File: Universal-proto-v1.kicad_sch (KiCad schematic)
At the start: 44 parts, among them J1 Bus_ISA_8bit, J2 ISA Breakout, J3 Pico GPIO Breakout

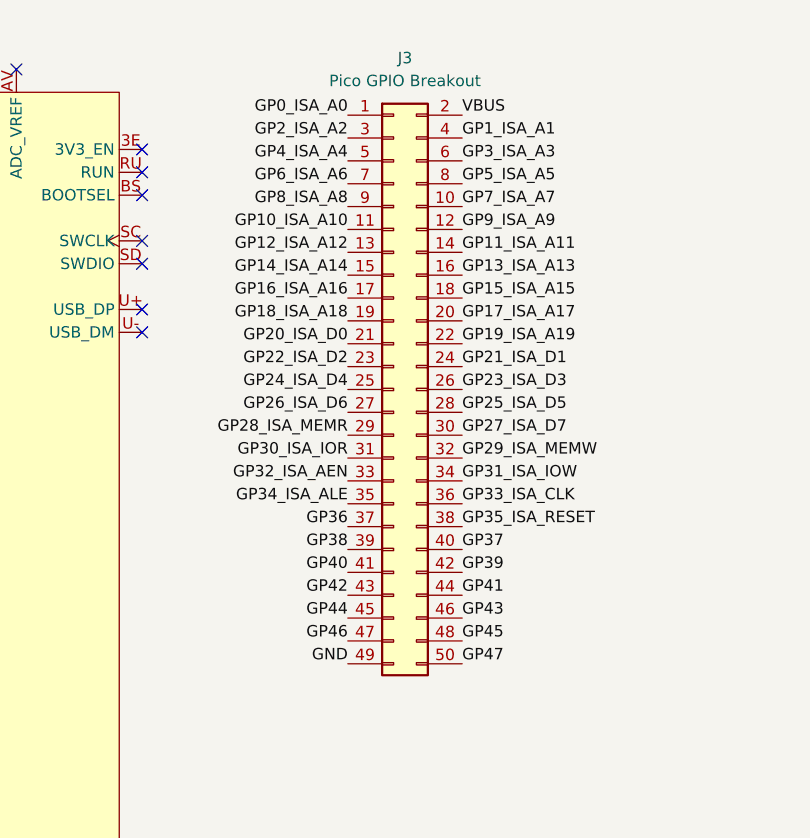
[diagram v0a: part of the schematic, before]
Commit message: Pre-split of GPIO breakout
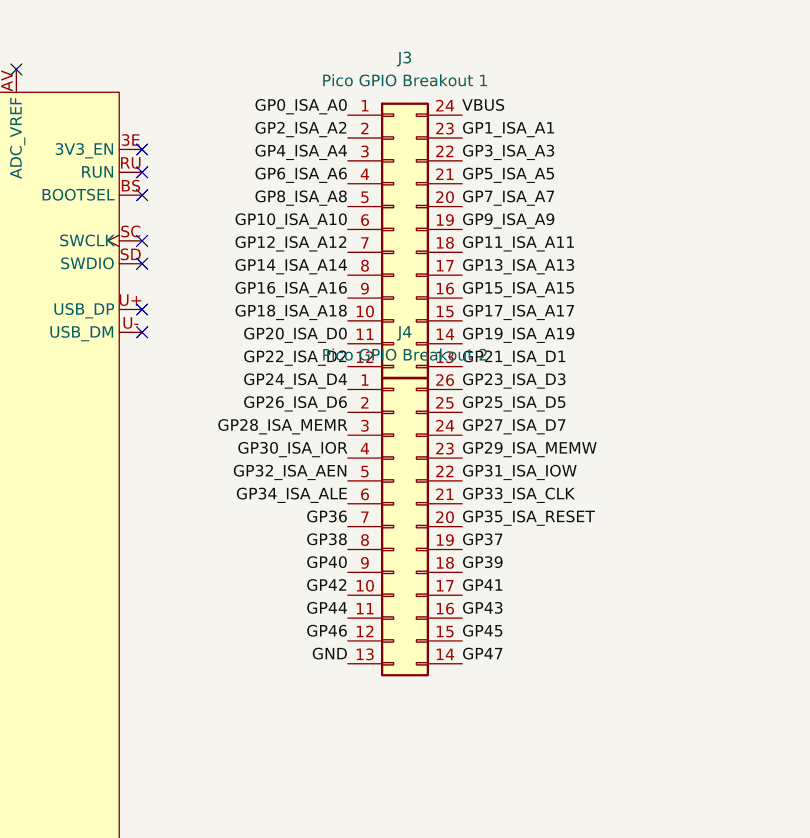
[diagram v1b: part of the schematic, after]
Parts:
- removed J3: Pico GPIO Breakout, Connector_PinHeader_2.54mm:PinHeader_2x25_P2.54mm_Vertical, symbol Connector_Generic:Conn_02x25_Odd_Even
- added J3: Pico GPIO Breakout 1, symbol Connector_Generic:Conn_02x12_Counter_Clockwise
- added J4: Pico GPIO Breakout 2, symbol Connector_Generic:Conn_02x13_Counter_Clockwise
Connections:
- net GND: now also J4.13 (Pin_13)
- net GP0_ISA_A0: now also J3.1 (Pin_1)
- net GP10_ISA_A10: now also J3.6 (Pin_6)
- net GP11_ISA_A11: now also J3.18 (Pin_18)
- net GP12_ISA_A12: now also J3.7 (Pin_7)
- net GP13_ISA_A13: now also J3.17 (Pin_17)
- net GP14_ISA_A14: now also J3.8 (Pin_8)
- net GP15_ISA_A15: now also J3.16 (Pin_16)
- net GP16_ISA_A16: now also J3.9 (Pin_9)
- net GP17_ISA_A17: now also J3.15 (Pin_15)
- net GP18_ISA_A18: now also J3.10 (Pin_10)
- net GP19_ISA_A19: now also J3.14 (Pin_14)
- net GP1_ISA_A1: now also J3.23 (Pin_23)
- net GP20_ISA_D0: now also J3.11 (Pin_11)
- net GP21_ISA_D1: now also J3.13 (Pin_13)
- net GP22_ISA_D2: now also J3.12 (Pin_12)
- net GP23_ISA_D3: now also J4.26 (Pin_26)
- net GP24_ISA_D4: now also J4.1 (Pin_1)
- net GP25_ISA_D5: now also J4.25 (Pin_25)
- net GP26_ISA_D6: now also J4.2 (Pin_2)
- net GP27_ISA_D7: now also J4.24 (Pin_24)
- net GP28_ISA_MEMR: now also J4.3 (Pin_3)
- net GP29_ISA_MEMW: now also J4.23 (Pin_23)
- net GP2_ISA_A2: now also J3.2 (Pin_2)
- net GP30_ISA_IOR: now also J4.4 (Pin_4)
- net GP31_ISA_IOW: now also J4.22 (Pin_22)
- net GP32_ISA_AEN: now also J4.5 (Pin_5)
- net GP33_ISA_CLK: now also J4.21 (Pin_21)
- net GP34_ISA_ALE: now also J4.6 (Pin_6)
- net GP35_ISA_RESET: now also J4.20 (Pin_20)
- net GP36: now also J4.7 (Pin_7)
- net GP37: now also J4.19 (Pin_19)
- net GP38: now also J4.8 (Pin_8)
- net GP39: now also J4.18 (Pin_18)
- net GP3_ISA_A3: now also J3.22 (Pin_22)
- net GP40: now also J4.9 (Pin_9)
- net GP41: now also J4.17 (Pin_17)
- net GP42: now also J4.10 (Pin_10)
- net GP43: now also J4.16 (Pin_16)
- net GP44: now also J4.11 (Pin_11)
- net GP45: now also J4.15 (Pin_15)
- net GP46: now also J4.12 (Pin_12)
- net GP47: now also J4.14 (Pin_14)
- net GP4_ISA_A4: now also J3.3 (Pin_3)
- net GP5_ISA_A5: now also J3.21 (Pin_21)
- net GP6_ISA_A6: now also J3.4 (Pin_4)
- net GP7_ISA_A7: now also J3.20 (Pin_20)
- net GP8_ISA_A8: now also J3.5 (Pin_5)
- net GP9_ISA_A9: now also J3.19 (Pin_19)
- net VBUS: now also J3.24 (Pin_24)
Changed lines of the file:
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@@
 	)
 	(symbol
+		(lib_id "Connector_Generic:Conn_02x13_Counter_Clockwise")
+		(at 229.87 71.12 0)
+		(unit 1)
+		(exclude_from_sim no)
+		(in_bom yes)
+		(on_board yes)
+		(dnp no)
+		(fields_autoplaced yes)
+		(property "Reference" "J4"
+			(at 231.14 49.53 0)
+			(effects
+				(font
+					(size 1.27 1.27)
+				)
+			)
+		)
+		(property "Value" "Pico GPIO Breakout 2"
+			(at 231.14 52.07 0)
+			(effects
+				(font
+					(size 1.27 1.27)
+				)
+			)
+		)
+		(property "Footprint" ""
+			(at 229.87 71.12 0)
+			(effects
+				(font
+					(size 1.27 1.27)
+				)
+				(hide yes)
+			)
+		)
+		(property "Datasheet" "~"
+			(at 229.87 71.12 0)
+			(effects
+				(font
+					(size 1.27 1.27)
+				)
+				(hide yes)
+			)
+		)
+		(property "Description" "Generic connector, double row, 02x13, counter clockwise pin numbering scheme (similar to DIP package numbering), script generated (kicad-library-utils/schlib/autogen/connector/)"
+			(at 229.87 71.12 0)
+			(effects
+				(font
+					(size 1.27 1.27)
+				)
+				(hide yes)
+			)
+		)
+		(pin "3"
+		)
+		(pin "4"
+		)
+		(pin "5"
+		)
+		(pin "6"
+		)
+		(pin "7"
+		)
+		(pin "8"
+		)
+		(pin "9"
+		)
+		(pin "10"
+		)
+		(pin "11"
+		)
+		(pin "12"
+		)
+		(pin "13"
+		)
+		(pin "26"
+		)
+		(pin "25"
+		)
+		(pin "24"
+		)
+		(pin "23"
+		)
+		(pin "22"
+		)
+		(pin "21"
+		)
+		(pin "20"
+		)
+		(pin "19"
+		)
+		(pin "18"
+		)
+		(pin "17"
+		)
+		(pin "16"
+		)
+		(pin "15"
+		)
+		(pin "14"
+		)
+		(pin "1"
+		)
+		(pin "2"
+		)
+		(instances
+			(project ""
+				(path "/14d49e36-dbe1-431d-b439-c2a0c8a95850"
+					(reference "J4")
+					(unit 1)
+				)
+			)
+		)
+	)
+	(symbol
 		(lib_id "Jumper:SolderJumper_2_Bridged")
 		(at 149.86 62.23 0)
@@
 	)
 	(symbol
-		(lib_id "Jumper:SolderJumper_2_Bridged")
-		(at 149.86 118.11 0)
+		(lib_id "Connector_Generic:Conn_02x12_Counter_Clockwise")
+		(at 229.87 38.1 0)
 		(unit 1)
 		(exclude_from_sim no)
-		(in_bom no)
+		(in_bom yes)
 		(on_board yes)
 		(dnp no)
 		(fields_autoplaced yes)
-		(property "Reference" "JP36"
-			(at 149.86 111.76 0)
+		(property "Reference" "J3"
+			(at 231.14 19.05 0)
 			(effects
 				(font
 					(size 1.27 1.27)
 				)
-				(hide yes)
 			)
 		)
-		(property "Value" "SolderJumper_2_Bridged"
-			(at 149.86 114.3 0)
+		(property "Value" "Pico GPIO Breakout 1"
+			(at 231.14 21.59 0)
 			(effects
 				(font
 					(size 1.27 1.27)
 				)
-				(hide yes)
 			)
 		)
-		(property "Footprint" "Jumper:SolderJumper-2_P1.3mm_Bridged_RoundedPad1.0x1.5mm"
-			(at 149.86 118.11 0)
+		(property "Footprint" ""
+			(at 229.87 38.1 0)
 			(effects
 				(font
@@
 		)
 		(property "Datasheet" "~"
-			(at 149.86 118.11 0)
+			(at 229.87 38.1 0)
 			(effects
 				(font
@@
 			)
 		)
-		(property "Description" "Solder Jumper, 2-pole, closed/bridged"
-			(at 149.86 118.11 0)
+		(property "Description" "Generic connector, double row, 02x12, counter clockwise pin numbering scheme (similar to DIP package numbering), script generated (kicad-library-utils/schlib/autogen/connector/)"
+			(at 229.87 38.1 0)
 			(effects
 				(font
@@
 			)
 		)
+		(pin "1"
+		)
 		(pin "2"
 		)
-		(pin "1"
+		(pin "3"
+		)
+		(pin "4"
+		)
+		(pin "5"
+		)
+		(pin "6"
+		)
+		(pin "7"
+		)
+		(pin "8"
+		)
+		(pin "9"
+		)
+		(pin "10"
+		)
+		(pin "11"
+		)
+		(pin "12"
+		)
+		(pin "24"
+		)
+		(pin "23"
+		)
+		(pin "22"
+		)
+		(pin "21"
+		)
+		(pin "20"
+		)
+		(pin "19"
+		)
+		(pin "18"
+		)
+		(pin "17"
+		)
+		(pin "16"
+		)
+		(pin "15"
+		)
+		(pin "14"
+		)
+		(pin "13"
 		)
 		(instances
-			(project "Universal-proto-v1"
+			(project ""
 				(path "/14d49e36-dbe1-431d-b439-c2a0c8a95850"
-					(reference "JP36")
+					(reference "J3")
 					(unit 1)
 				)
@@
 	)
 	(symbol
-		(lib_id "Connector_Generic:Conn_02x25_Odd_Even")
-		(at 229.87 55.88 0)
+		(lib_id "Jumper:SolderJumper_2_Bridged")
+		(at 149.86 118.11 0)
 		(unit 1)
 		(exclude_from_sim no)
-		(in_bom yes)
+		(in_bom no)
 		(on_board yes)
 		(dnp no)
 		(fields_autoplaced yes)
-		(property "Reference" "J3"
-			(at 231.14 19.05 0)
+		(property "Reference" "JP36"
+			(at 149.86 111.76 0)
 			(effects
 				(font
 					(size 1.27 1.27)
 				)
+				(hide yes)
 			)
 		)
-		(property "Value" "Pico GPIO Breakout"
-			(at 231.14 21.59 0)
+		(property "Value" "SolderJumper_2_Bridged"
+			(at 149.86 114.3 0)
 			(effects
 				(font
 					(size 1.27 1.27)
 				)
+				(hide yes)
 			)
 		)
-		(property "Footprint" "Connector_PinHeader_2.54mm:PinHeader_2x25_P2.54mm_Vertical"
-			(at 229.87 55.88 0)
+		(property "Footprint" "Jumper:SolderJumper-2_P1.3mm_Bridged_RoundedPad1.0x1.5mm"
+			(at 149.86 118.11 0)
 			(effects
 				(font
@@
 		)
 		(property "Datasheet" "~"
-			(at 229.87 55.88 0)
+			(at 149.86 118.11 0)
 			(effects
 				(font
@@
 			)
 		)
-		(property "Description" "Generic connector, double row, 02x25, odd/even pin numbering scheme (row 1 odd numbers, row 2 even numbers), script generated (kicad-library-utils/schlib/autogen/connector/)"
-			(at 229.87 55.88 0)
+		(property "Description" "Solder Jumper, 2-pole, closed/bridged"
+			(at 149.86 118.11 0)
 			(effects
 				(font
@@
 			)
 		)
-		(pin "1"
-		)
-		(pin "3"
-		)
-		(pin "5"
-		)
-		(pin "7"
-		)
-		(pin "9"
-		)
-		(pin "11"
-		)
-		(pin "13"
-		)
-		(pin "15"
-		)
-		(pin "17"
-		)
-		(pin "19"
-		)
-		(pin "21"
-		)
-		(pin "23"
-		)
-		(pin "25"
-		)
-		(pin "27"
-		)
-		(pin "29"
-		)
-		(pin "31"
-		)
-		(pin "33"
-		)
-		(pin "35"
-		)
-		(pin "37"
-		)
-		(pin "39"
-		)
-		(pin "41"
-		)
-		(pin "43"
-		)
-		(pin "45"
-		)
-		(pin "47"
-		)
-		(pin "49"
-		)
 		(pin "2"
 		)
-		(pin "4"
-		)
-		(pin "6"
-		)
-		(pin "8"
-		)
-		(pin "10"
-		)
-		(pin "12"
-		)
-		(pin "14"
-		)
-		(pin "16"
-		)
-		(pin "18"
-		)
-		(pin "20"
-		)
-		(pin "22"
-		)
-		(pin "24"
-		)
-		(pin "26"
-		)
-		(pin "28"
-		)
-		(pin "30"
-		)
-		(pin "32"
-		)
-		(pin "34"
-		)
-		(pin "36"
-		)
-		(pin "38"
-		)
-		(pin "40"
-		)
-		(pin "42"
-		)
-		(pin "44"
-		)
-		(pin "46"
-		)
-		(pin "48"
-		)
-		(pin "50"
+		(pin "1"
 		)
 		(instances
-			(project ""
+			(project "Universal-proto-v1"
 				(path "/14d49e36-dbe1-431d-b439-c2a0c8a95850"
-					(reference "J3")
+					(reference "JP36")
 					(unit 1)
 				)

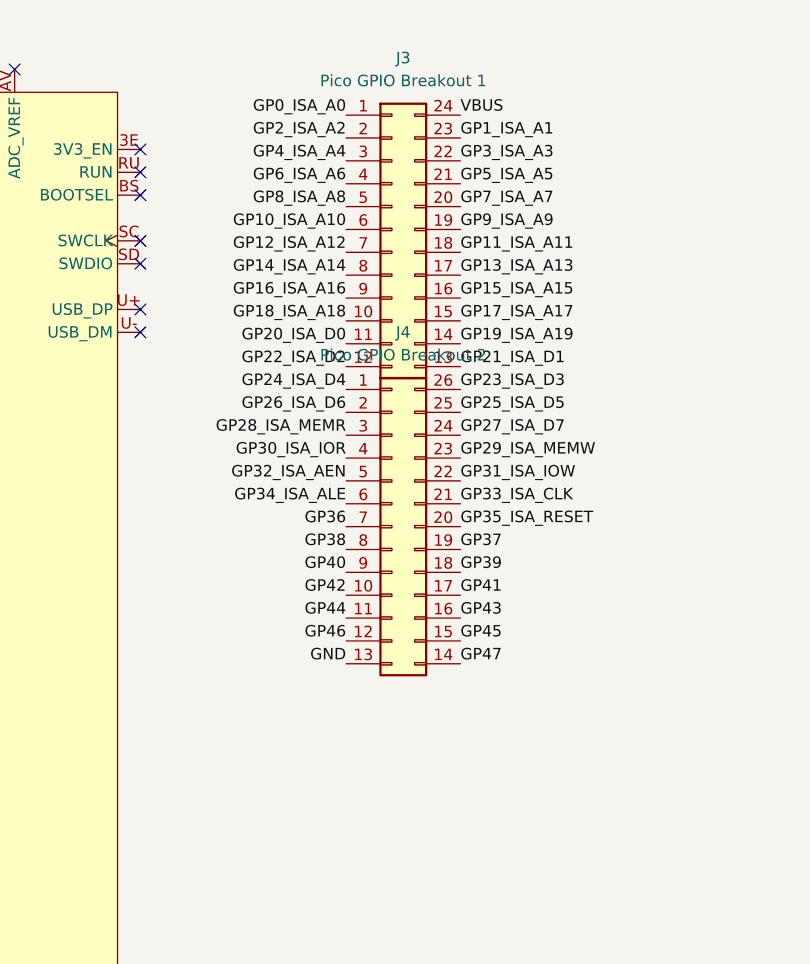
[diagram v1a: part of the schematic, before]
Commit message: Everything seems to fit
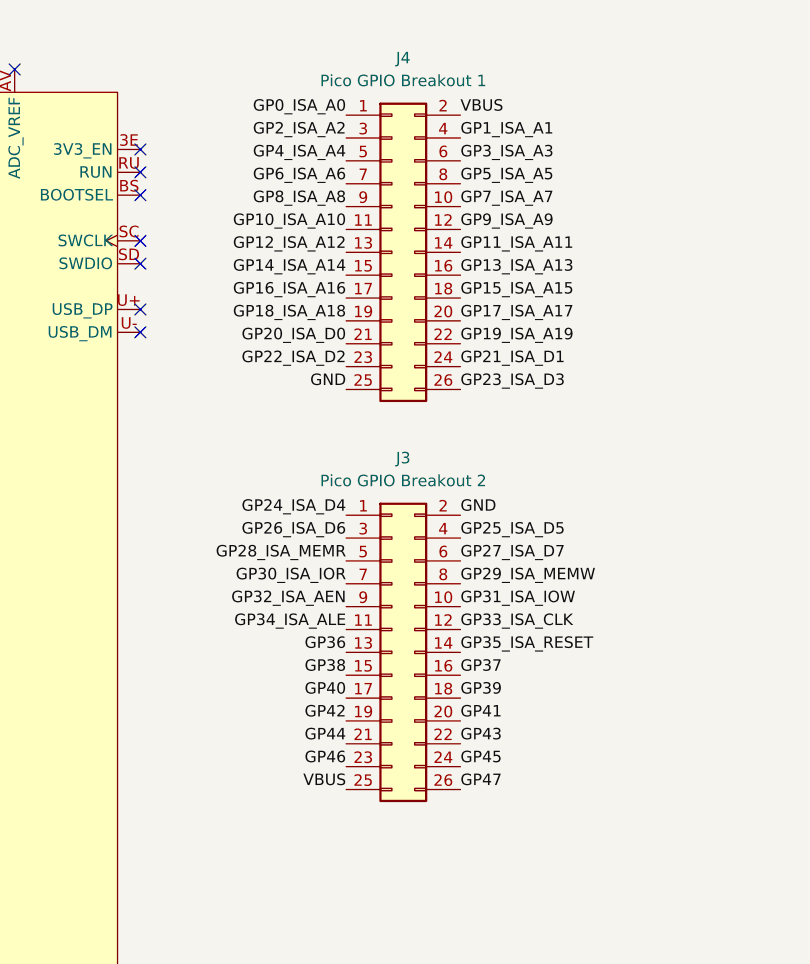
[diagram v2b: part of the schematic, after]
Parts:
- removed J3: Pico GPIO Breakout 1, symbol Connector_Generic:Conn_02x12_Counter_Clockwise
- removed J4: Pico GPIO Breakout 2, symbol Connector_Generic:Conn_02x13_Counter_Clockwise
- added J3: Pico GPIO Breakout 2, Connector_PinHeader_2.54mm:PinHeader_2x13_P2.54mm_Vertical, symbol Connector_Generic:Conn_02x13_Odd_Even
- added J4: Pico GPIO Breakout 1, Connector_PinHeader_2.54mm:PinHeader_2x13_P2.54mm_Vertical, symbol Connector_Generic:Conn_02x13_Odd_Even
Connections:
- net GND: now also J3.2 (Pin_2), J4.25 (Pin_25)
- net GP0_ISA_A0: now also J4.1 (Pin_1)
- net GP10_ISA_A10: now also J4.11 (Pin_11)
- net GP11_ISA_A11: now also J4.14 (Pin_14)
- net GP12_ISA_A12: now also J4.13 (Pin_13)
- net GP13_ISA_A13: now also J4.16 (Pin_16)
- net GP14_ISA_A14: now also J4.15 (Pin_15)
- net GP15_ISA_A15: now also J4.18 (Pin_18)
- net GP16_ISA_A16: now also J4.17 (Pin_17)
- net GP17_ISA_A17: now also J4.20 (Pin_20)
- net GP18_ISA_A18: now also J4.19 (Pin_19)
- net GP19_ISA_A19: now also J4.22 (Pin_22)
- net GP1_ISA_A1: now also J4.4 (Pin_4)
- net GP20_ISA_D0: now also J4.21 (Pin_21)
- net GP21_ISA_D1: now also J4.24 (Pin_24)
- net GP22_ISA_D2: now also J4.23 (Pin_23)
- net GP23_ISA_D3: now also J4.26 (Pin_26)
- net GP24_ISA_D4: now also J3.1 (Pin_1)
- net GP25_ISA_D5: now also J3.4 (Pin_4)
- net GP26_ISA_D6: now also J3.3 (Pin_3)
- net GP27_ISA_D7: now also J3.6 (Pin_6)
- net GP28_ISA_MEMR: now also J3.5 (Pin_5)
- net GP29_ISA_MEMW: now also J3.8 (Pin_8)
- net GP2_ISA_A2: now also J4.3 (Pin_3)
- net GP30_ISA_IOR: now also J3.7 (Pin_7)
- net GP31_ISA_IOW: now also J3.10 (Pin_10)
- net GP32_ISA_AEN: now also J3.9 (Pin_9)
- net GP33_ISA_CLK: now also J3.12 (Pin_12)
- net GP34_ISA_ALE: now also J3.11 (Pin_11)
- net GP35_ISA_RESET: now also J3.14 (Pin_14)
- net GP36: now also J3.13 (Pin_13)
- net GP37: now also J3.16 (Pin_16)
- net GP38: now also J3.15 (Pin_15)
- net GP39: now also J3.18 (Pin_18)
- net GP3_ISA_A3: now also J4.6 (Pin_6)
- net GP40: now also J3.17 (Pin_17)
- net GP41: now also J3.20 (Pin_20)
- net GP42: now also J3.19 (Pin_19)
- net GP43: now also J3.22 (Pin_22)
- net GP44: now also J3.21 (Pin_21)
- net GP45: now also J3.24 (Pin_24)
- net GP46: now also J3.23 (Pin_23)
- net GP47: now also J3.26 (Pin_26)
- net GP4_ISA_A4: now also J4.5 (Pin_5)
- net GP5_ISA_A5: now also J4.8 (Pin_8)
- net GP6_ISA_A6: now also J4.7 (Pin_7)
- net GP7_ISA_A7: now also J4.10 (Pin_10)
- net GP8_ISA_A8: now also J4.9 (Pin_9)
- net GP9_ISA_A9: now also J4.12 (Pin_12)
- net VBUS: now also J3.25 (Pin_25), J4.2 (Pin_2)
